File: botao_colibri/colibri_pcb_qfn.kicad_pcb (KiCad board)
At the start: 2 copper layers, 72.5 x 47.1 mm, 39 parts, among them J1 USB4970-00-A_REVA, J2 TC2030, J3 Conn_01x02, J4 PJ-307C, SW1 B3F-3122, U1 ME54BS12, U4 NPM1300-QEAA-R7

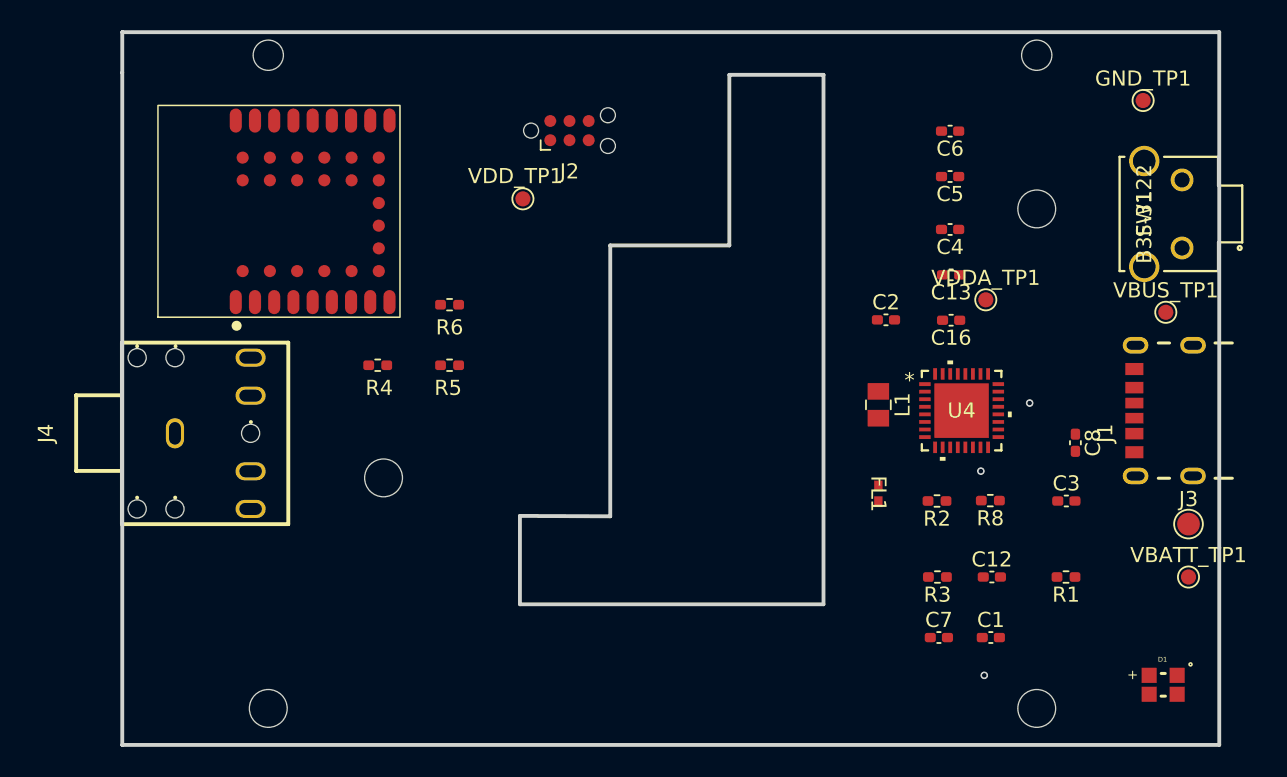
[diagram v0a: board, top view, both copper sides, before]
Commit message: Trilhas feitas
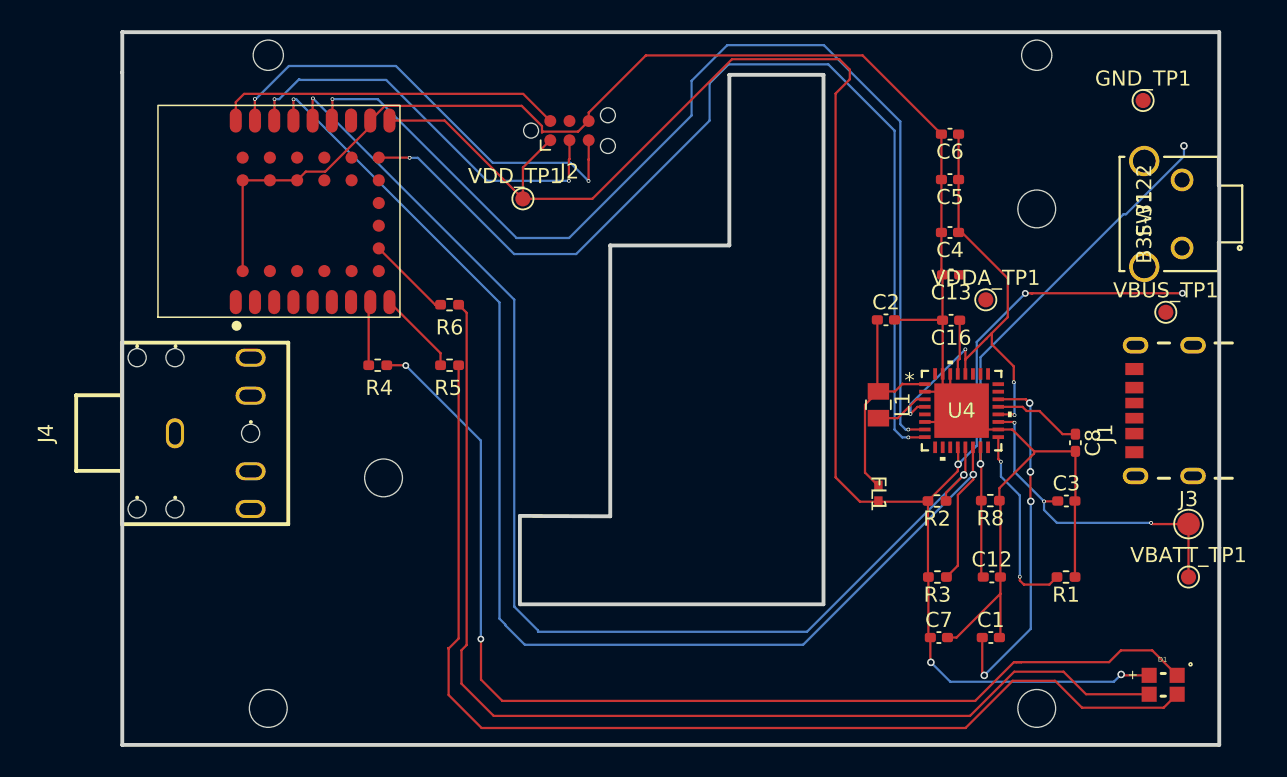
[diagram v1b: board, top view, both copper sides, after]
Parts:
- moved C4 0.20 mm to (178.7, 85.7)
- moved C5 0.20 mm to (178.7, 82.2)
- moved C6 0.20 mm to (178.7, 79.2)
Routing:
- net VDD: track 0.00 -> 129.6 mm, vias 0 -> 5
- net GND: track 0.00 -> 124.6 mm
- net I2C_SCL: track 0.00 -> 87.5 mm, vias 0 -> 2
- net I2C_SDA: track 0.00 -> 79.4 mm, vias 0 -> 2
- net Net-(D1-Pad2): track 0.00 -> 73.6 mm
- net Net-(D1-Pad3): track 0.00 -> 73.6 mm
- net NPM1300_INT: track 0.00 -> 73.3 mm, vias 0 -> 2
- net Net-(D1-Pad1): track 0.00 -> 73.2 mm, vias 0 -> 2
- net NPM1300_EN: track 0.00 -> 67.2 mm, vias 0 -> 2
- net BTN_PWR: track 0.00 -> 35.3 mm, vias 0 -> 2
- net PVDD: track 0.00 -> 33.3 mm, vias 0 -> 4
- net SWCLK: track 0.00 -> 30.2 mm, vias 0 -> 2
- net SWDIO: track 0.00 -> 26.9 mm, vias 0 -> 2
- net Net-(U4-VBUSOUT): track 0.00 -> 24.0 mm, vias 0 -> 4
- net NRESET: track 0.00 -> 23.0 mm
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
